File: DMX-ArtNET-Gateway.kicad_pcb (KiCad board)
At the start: 2 copper layers, 91.4 x 55.9 mm, 45 parts, among them J1 GPIO Breakout, J2 DMX1, J3 DMX2, J4 Barrel_Jack_MountingPin, U1 AMS1117-3.3, U2 ESP32-WROOM-32D, U3 MAX485CSA, U4 MAX485CSA

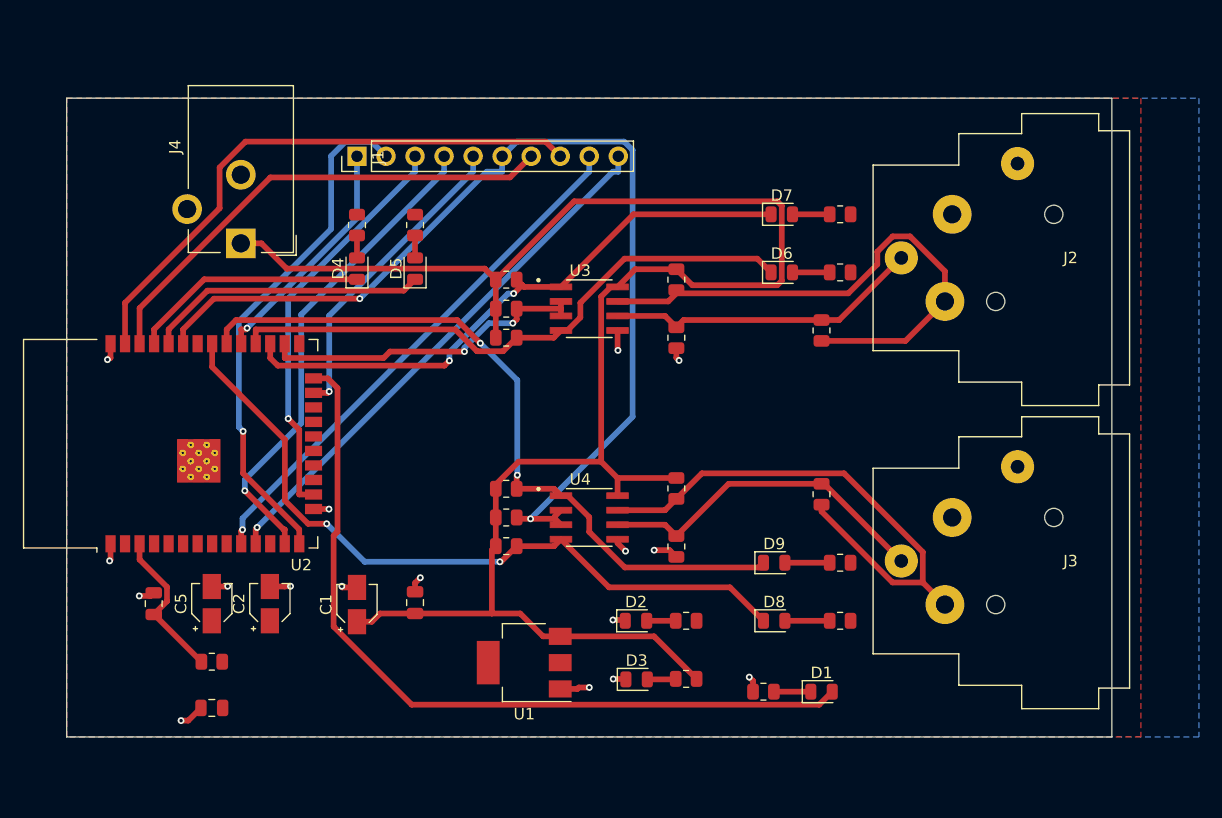
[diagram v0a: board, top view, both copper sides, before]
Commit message: Firmware checkin
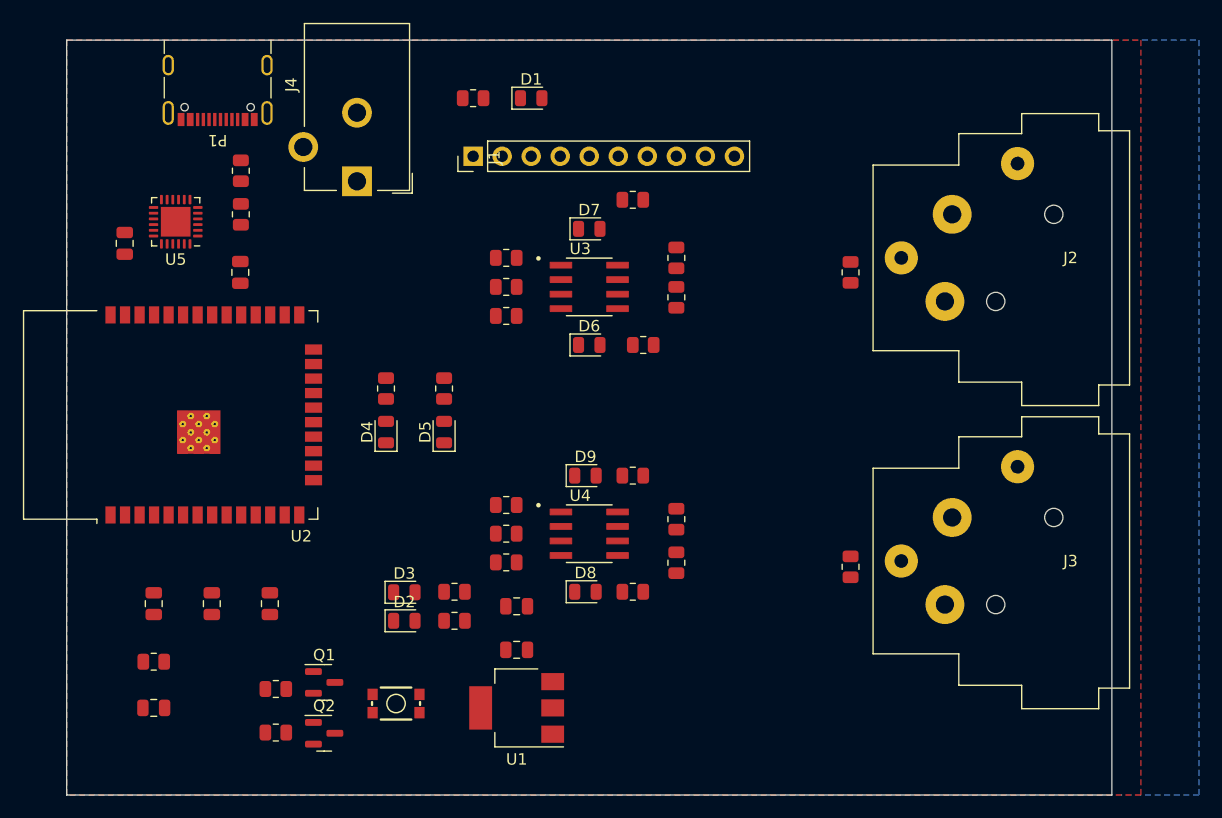
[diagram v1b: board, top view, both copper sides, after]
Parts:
- added C7: 10uF, SparkFun-Capacitor:C_0805_2012Metric, F.Cu at (119.4, 94.0)
- added C8: 1uF, SparkFun-Capacitor:C_0805_2012Metric, F.Cu at (129.5, 96.5)
- added P1: USB_C_Plug_USB2.0, Connector_USB:USB_C_Receptacle_GCT_USB4105-xx-A_16P_TopMnt_Horizontal, F.Cu at (127.5, 79.5)
- added Q1: MMBT3904, Package_TO_SOT_SMD:SOT-23, F.Cu at (136.8, 132.4)
- added Q2: MMBT3904, Package_TO_SOT_SMD:SOT-23, F.Cu at (136.8, 136.8)
- added R23: 10K, SparkFun-Resistor:R_0805_2012Metric, F.Cu at (129.5, 87.6)
- added R24: 20K, SparkFun-Resistor:R_0805_2012Metric, F.Cu at (129.5, 91.4)
- added R25: 10K, SparkFun-Resistor:R_0805_2012Metric, F.Cu at (132.6, 136.8)
- added R26: 10K, SparkFun-Resistor:R_0805_2012Metric, F.Cu at (132.6, 133.0)
- added SW1: Reset, SparkFun-Switch:Momentary_SMD_4.6x2.8mm, F.Cu at (143.1, 134.2)
- added U5: CP2104, Package_DFN_QFN:QFN-24-1EP_4x4mm_P0.5mm_EP2.6x2.6mm, F.Cu at (123.8, 92.1)
- C1, C2, C5: footprint Capacitor_SMD:CP_Elec_3x5.3 -> SparkFun-Capacitor:C_0805_2012Metric
- R10: value 1k -> 10k
- moved D1 57.8 mm to (154.9, 81.3)
- moved R1 57.8 mm to (149.9, 81.3)
- moved D3 21.7 mm to (143.8, 124.5)
- moved R3 21.7 mm to (148.2, 124.5)
- moved R2 20.3 mm to (148.2, 127.0)
- moved D2 20.3 mm to (143.8, 127.0)
- moved R9 19.7 mm to (163.8, 114.3)
- moved R6 18.4 mm to (164.7, 102.9)
- moved R8 18.3 mm to (163.8, 124.5)
- moved D9 18.2 mm to (159.7, 114.3)
- moved R7 18.2 mm to (163.8, 90.2)
- moved D6 18.0 mm to (160.0, 102.9)
- moved D7 16.9 mm to (160.0, 92.7)
- moved D8 16.7 mm to (159.7, 124.5)
- moved R4 14.5 mm to (142.2, 106.7)
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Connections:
- net Net-(U2-EN) renamed CHIP_PU
- U2 pad 25: unconnected-(U2-IO0-Pad25) -> IO0
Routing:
- net +5V: track 157.8 -> 0.00 mm
- net IO21: track 89.5 -> 0.00 mm, vias 2 -> 0
- net IO2: track 70.4 -> 0.00 mm
- net IO19: track 64.2 -> 0.00 mm, vias 2 -> 0
- net IO18: track 64.1 -> 0.00 mm, vias 2 -> 0
- net IO16: track 52.1 -> 0.00 mm, vias 2 -> 0
- net IO17: track 51.7 -> 0.00 mm
- net IO23: track 50.1 -> 0.00 mm
- net DMX_2_B: track 48.3 -> 0.00 mm
- net DMX_1_B: track 48.1 -> 0.00 mm
- net IO26: track 47.3 -> 0.00 mm, vias 1 -> 0
- net IO25: track 46.5 -> 0.00 mm, vias 1 -> 0
- net IO12: track 45.3 -> 0.00 mm, vias 1 -> 0
- net IO22: track 42.9 -> 0.00 mm
- net IO14: track 42.6 -> 0.00 mm, vias 1 -> 0
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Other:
- board size 91.4 x 55.9 mm -> 91.4 x 66 mm
